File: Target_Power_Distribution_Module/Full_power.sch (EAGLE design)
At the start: 26 parts, among them IC1 MCP1702, Q1 NFET, Q2 PFET, Q3 NFET, Q4 PFET

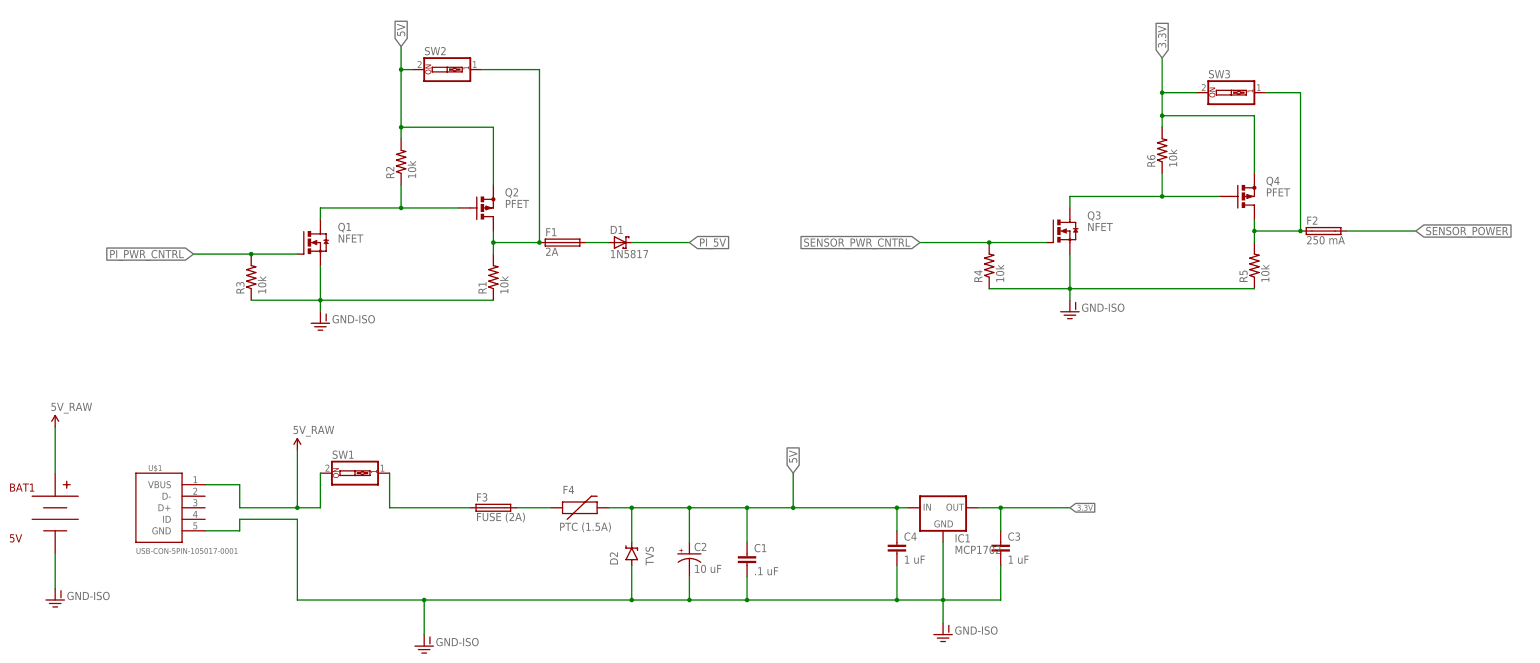
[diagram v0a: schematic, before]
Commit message: Started on brd
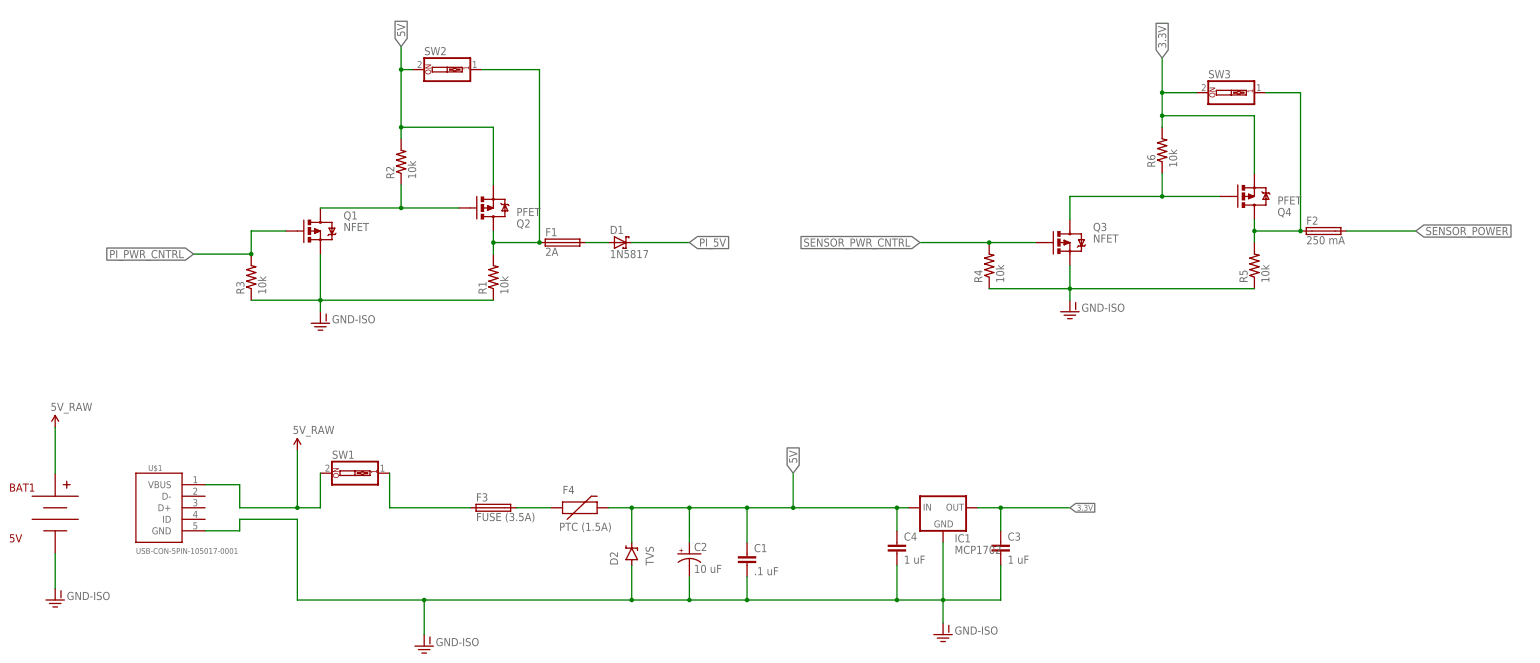
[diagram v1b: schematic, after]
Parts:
- F3: value FUSE (2A) -> FUSE (3.5A); device fuse:FUSE1821 -> fuse:PICOFUSE
- Q1, Q3: device transistor-power:IRF3704 -> User-Submitted:MOSFET-PCHANNELFQP27P06
- Q2, Q4: device adafruit:PFETBS250 -> User-Submitted:MOSFET-PCHANNELFQP27P06
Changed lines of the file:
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@@
 </classes>
 <parts>
-<part name="Q1" library="transistor-power" deviceset="IRF3704" device="" value="NFET"/>
-<part name="Q2" library="adafruit" deviceset="PFET" device="BS250" value="PFET"/>
+<part name="Q1" library="User-Submitted" deviceset="MOSFET-PCHANNEL" device="FQP27P06" value="NFET"/>
+<part name="Q2" library="User-Submitted" deviceset="MOSFET-PCHANNEL" device="FQP27P06" value="PFET"/>
 <part name="GND-ISO1" library="SparkFun-Aesthetics" deviceset="GND-ISO" device=""/>
 <part name="R1" library="SparkFun-Resistors" deviceset="RESISTOR" device="1206" value="10k"/>
@@
 <part name="D1" library="adafruit" deviceset="SCHOTTKY-DIODE" device="CB429-15" value="1N5817"/>
 <part name="F1" library="fuse" deviceset="FUSE" device="PICOFUSE" value="2A"/>
-<part name="Q3" library="transistor-power" deviceset="IRF3704" device="" value="NFET"/>
-<part name="Q4" library="adafruit" deviceset="PFET" device="BS250" value="PFET"/>
+<part name="Q3" library="User-Submitted" deviceset="MOSFET-PCHANNEL" device="FQP27P06" value="NFET"/>
+<part name="Q4" library="User-Submitted" deviceset="MOSFET-PCHANNEL" device="FQP27P06" value="PFET"/>
 <part name="F2" library="fuse" deviceset="FUSE" device="PICOFUSE" value="250 mA"/>
 <part name="R4" library="SparkFun-Resistors" deviceset="RESISTOR" device="1206" value="10k"/>
@@
 <part name="U$1" library="GeekAmmo" deviceset="USB-CON-5PIN" device="-105017-0001"/>
 <part name="D2" library="SparkFun-DiscreteSemi" deviceset="DIODE-ZENER" device="PTH" value="TVS"/>
-<part name="F3" library="fuse" deviceset="FUSE" device="1821" value="FUSE (2A)"/>
+<part name="F3" library="fuse" deviceset="PICOFUSE" device="" value="FUSE (3.5A)"/>
 <part name="F4" library="SparkFun-PowerIC" deviceset="PTC" device="PTH" value="PTC (1.5A)"/>
 <part name="C1" library="SparkFun-Capacitors" deviceset="CAP" device="1206" value=".1 uF"/>
@@
 </plain>
 <instances>
-<instance part="Q1" gate="G$1" x="-182.88" y="30.48"/>
-<instance part="Q2" gate="1" x="-144.78" y="38.1"/>
+<instance part="Q1" gate="G$1" x="-180.34" y="33.02"/>
+<instance part="Q2" gate="G$1" x="-142.24" y="38.1" rot="MR180"/>
 <instance part="GND-ISO1" gate="G$1" x="-180.34" y="12.7"/>
 <instance part="R1" gate="G$1" x="-142.24" y="22.86" rot="R90"/>
@@
 <instance part="D1" gate="G$1" x="-114.3" y="30.48"/>
 <instance part="F1" gate="G$1" x="-127" y="30.48"/>
-<instance part="Q3" gate="G$1" x="-17.78" y="33.02"/>
-<instance part="Q4" gate="1" x="22.86" y="40.64"/>
+<instance part="Q3" gate="G$1" x="-15.24" y="30.48"/>
+<instance part="Q4" gate="G$1" x="25.4" y="40.64" rot="MR180"/>
 <instance part="F2" gate="G$1" x="40.64" y="33.02"/>
 <instance part="R4" gate="G$1" x="-33.02" y="25.4" rot="R90"/>
@@
 <attribute name="VALUE" x="-106.9086" y="-40.64" size="1.778" layer="96" rot="R90"/>
 </instance>
-<instance part="F3" gate="G$1" x="-142.24" y="-27.94"/>
+<instance part="F3" gate="1" x="-142.24" y="-27.94"/>
 <instance part="F4" gate="G$1" x="-124.46" y="-27.94"/>
 <instance part="C1" gate="G$1" x="-86.36" y="-40.64"/>
@@
 <pinref part="Q1" gate="G$1" pin="S"/>
 <pinref part="GND-ISO1" gate="G$1" pin="GND-ISO"/>
-<wire x1="-180.34" y1="25.4" x2="-180.34" y2="17.78" width="0.1524" layer="91"/>
+<wire x1="-180.34" y1="27.94" x2="-180.34" y2="17.78" width="0.1524" layer="91"/>
 <pinref part="R3" gate="G$1" pin="1"/>
 <wire x1="-180.34" y1="17.78" x2="-180.34" y2="15.24" width="0.1524" layer="91"/>
@@
 <junction x="-15.24" y="20.32"/>
 <pinref part="Q3" gate="G$1" pin="S"/>
-<wire x1="-15.24" y1="27.94" x2="-15.24" y2="20.32" width="0.1524" layer="91"/>
+<wire x1="-15.24" y1="25.4" x2="-15.24" y2="20.32" width="0.1524" layer="91"/>
 </segment>
 <segment>
@@
 <segment>
 <pinref part="Q1" gate="G$1" pin="D"/>
-<wire x1="-180.34" y1="35.56" x2="-180.34" y2="38.1" width="0.1524" layer="91"/>
-<pinref part="Q2" gate="1" pin="G"/>
+<pinref part="Q2" gate="G$1" pin="G"/>
 <wire x1="-180.34" y1="38.1" x2="-162.56" y2="38.1" width="0.1524" layer="91"/>
 <pinref part="R2" gate="G$1" pin="1"/>
@@
 <segment>
 <pinref part="R3" gate="G$1" pin="2"/>
+<wire x1="-195.58" y1="27.94" x2="-208.28" y2="27.94" width="0.1524" layer="91"/>
+<label x="-208.28" y="27.94" size="1.778" layer="95" rot="R180" xref="yes"/>
+<wire x1="-195.58" y1="27.94" x2="-195.58" y2="33.02" width="0.1524" layer="91"/>
+<junction x="-195.58" y="27.94"/>
 <pinref part="Q1" gate="G$1" pin="G"/>
-<wire x1="-195.58" y1="27.94" x2="-185.42" y2="27.94" width="0.1524" layer="91"/>
-<wire x1="-195.58" y1="27.94" x2="-208.28" y2="27.94" width="0.1524" layer="91"/>
-<junction x="-195.58" y="27.94"/>
-<label x="-208.28" y="27.94" size="1.778" layer="95" rot="R180" xref="yes"/>
+<wire x1="-195.58" y1="33.02" x2="-187.96" y2="33.02" width="0.1524" layer="91"/>
 </segment>
 </net>
@@
 <segment>
 <pinref part="R1" gate="G$1" pin="2"/>
-<pinref part="Q2" gate="1" pin="D"/>
+<pinref part="Q2" gate="G$1" pin="D"/>
 <wire x1="-142.24" y1="27.94" x2="-142.24" y2="30.48" width="0.1524" layer="91"/>
 <pinref part="F1" gate="G$1" pin="1"/>
@@
 <net name="N$1" class="0">
 <segment>
-<pinref part="Q4" gate="1" pin="G"/>
+<pinref part="Q4" gate="G$1" pin="G"/>
 <pinref part="R6" gate="G$1" pin="1"/>
 <wire x1="17.78" y1="40.64" x2="5.08" y2="40.64" width="0.1524" layer="91"/>
 <wire x1="5.08" y1="40.64" x2="5.08" y2="45.72" width="0.1524" layer="91"/>
 <pinref part="Q3" gate="G$1" pin="D"/>
-<wire x1="-15.24" y1="38.1" x2="-15.24" y2="40.64" width="0.1524" layer="91"/>
+<wire x1="-15.24" y1="35.56" x2="-15.24" y2="40.64" width="0.1524" layer="91"/>
 <wire x1="-15.24" y1="40.64" x2="5.08" y2="40.64" width="0.1524" layer="91"/>
 <junction x="5.08" y="40.64"/>
@@
 <net name="3.3V" class="0">
 <segment>
-<pinref part="Q4" gate="1" pin="S"/>
+<pinref part="Q4" gate="G$1" pin="S"/>
 <wire x1="25.4" y1="45.72" x2="25.4" y2="58.42" width="0.1524" layer="91"/>
 <wire x1="25.4" y1="58.42" x2="5.08" y2="58.42" width="0.1524" layer="91"/>
@@
 <net name="5V" class="0">
 <segment>
-<pinref part="Q2" gate="1" pin="S"/>
+<pinref part="Q2" gate="G$1" pin="S"/>
 <wire x1="-142.24" y1="43.18" x2="-142.24" y2="55.88" width="0.1524" layer="91"/>
 <wire x1="-142.24" y1="55.88" x2="-162.56" y2="55.88" width="0.1524" layer="91"/>
@@
 <pinref part="R4" gate="G$1" pin="2"/>
 <pinref part="Q3" gate="G$1" pin="G"/>
-<wire x1="-33.02" y1="30.48" x2="-20.32" y2="30.48" width="0.1524" layer="91"/>
+<wire x1="-33.02" y1="30.48" x2="-22.86" y2="30.48" width="0.1524" layer="91"/>
 <wire x1="-33.02" y1="30.48" x2="-48.26" y2="30.48" width="0.1524" layer="91"/>
 <junction x="-33.02" y="30.48"/>
@@
 <net name="N$6" class="0">
 <segment>
-<pinref part="Q4" gate="1" pin="D"/>
+<pinref part="Q4" gate="G$1" pin="D"/>
 <pinref part="R5" gate="G$1" pin="2"/>
 <wire x1="25.4" y1="35.56" x2="25.4" y2="33.02" width="0.1524" layer="91"/>
@@
 <net name="N$7" class="0">
 <segment>
-<pinref part="F3" gate="G$1" pin="2"/>
+<pinref part="F3" gate="1" pin="2"/>
 <pinref part="F4" gate="G$1" pin="1"/>
 <wire x1="-137.16" y1="-27.94" x2="-129.54" y2="-27.94" width="0.1524" layer="91"/>
@@
 <net name="5V_SWITCH" class="0">
 <segment>
-<pinref part="F3" gate="G$1" pin="1"/>
+<pinref part="F3" gate="1" pin="1"/>
 <wire x1="-147.32" y1="-27.94" x2="-165.1" y2="-27.94" width="0.1524" layer="91"/>
 <pinref part="SW1" gate="G$1" pin="1"/>
